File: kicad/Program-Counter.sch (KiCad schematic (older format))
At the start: 6 parts, among them U89 74LS161, U90 74LS245, U91 74LS161, U92 74LS245, U93 74LS161, U94 74LS161

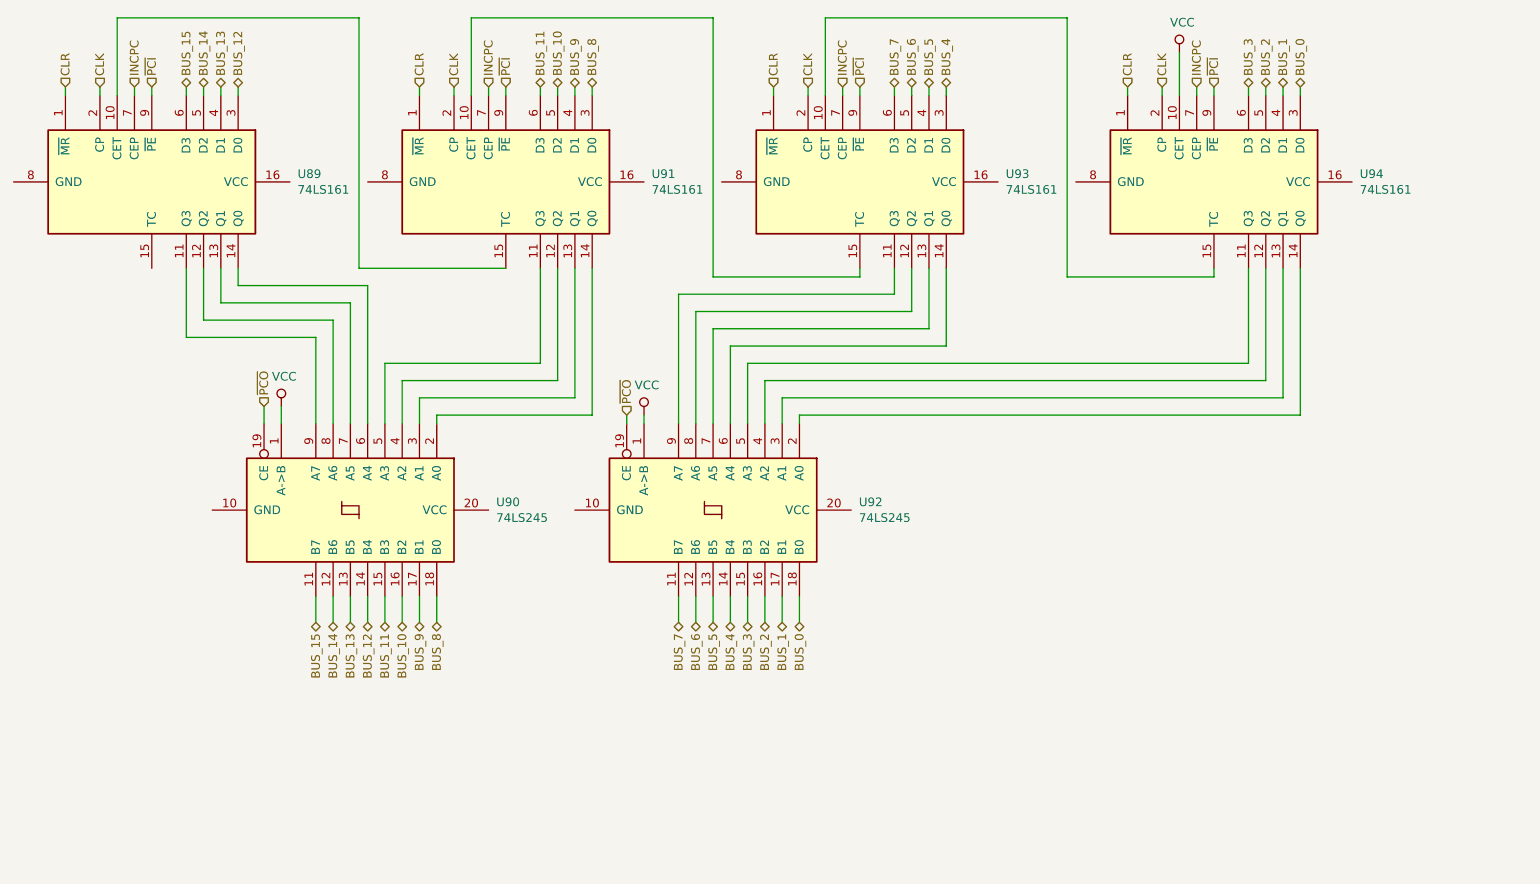
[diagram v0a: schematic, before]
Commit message: Up to v1.0 and plot
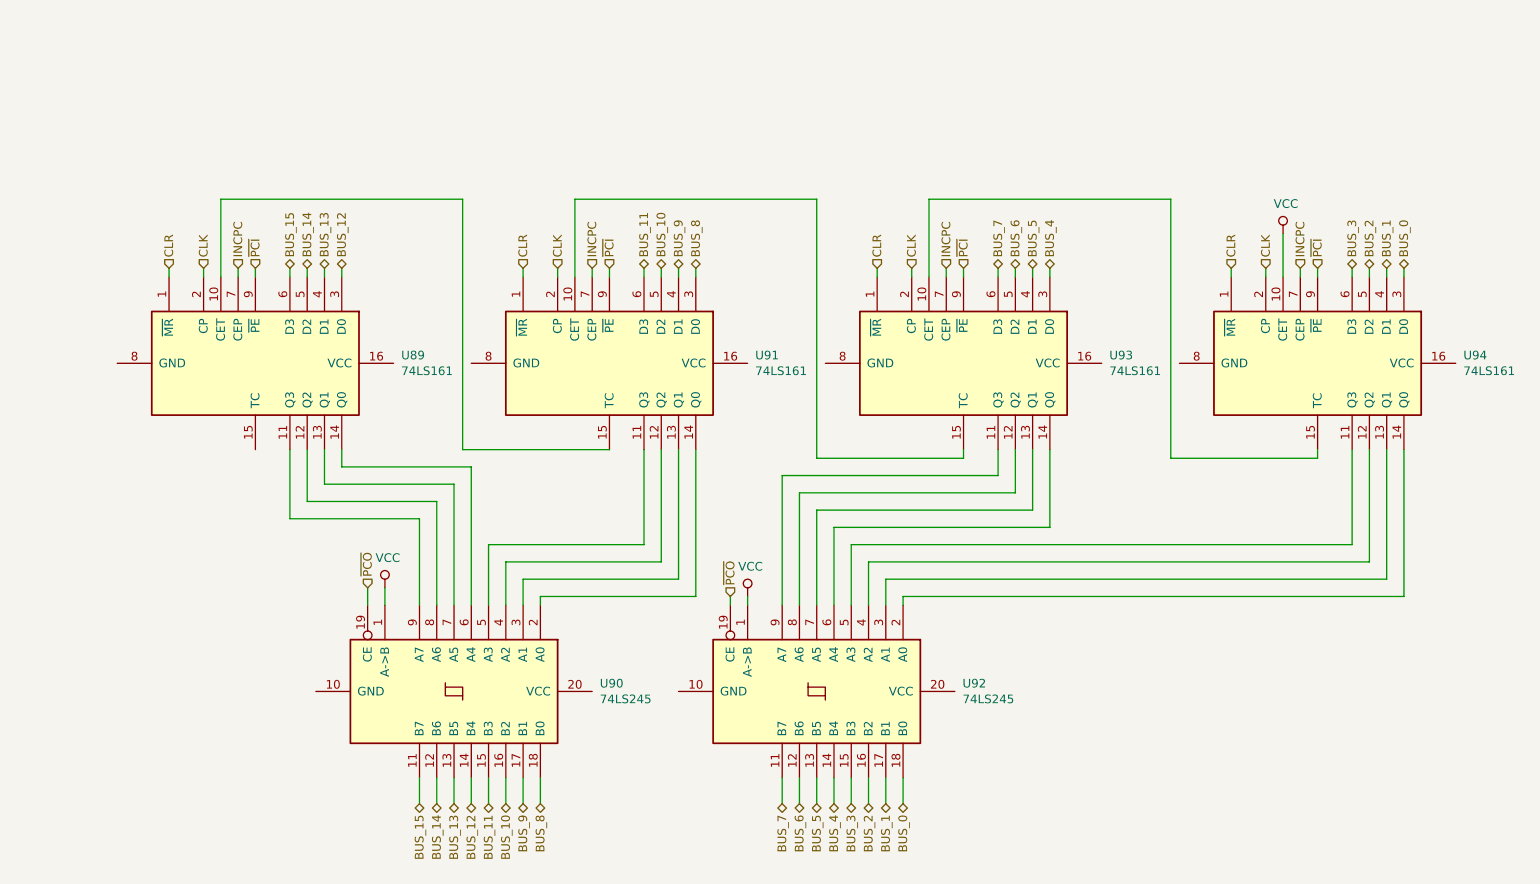
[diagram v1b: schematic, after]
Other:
- moved on the sheet: U89, U90, U91, U92, U93, U94
